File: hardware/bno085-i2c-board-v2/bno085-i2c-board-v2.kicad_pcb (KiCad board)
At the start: 2 copper layers, 13 parts, among them J1 Conn_01x01_Pin, J2 Conn_01x01_Pin, J3 Conn_01x01_Pin, J4 Conn_01x01_Pin, J5 Conn_01x01_Pin, J6 Conn_01x01_Pin

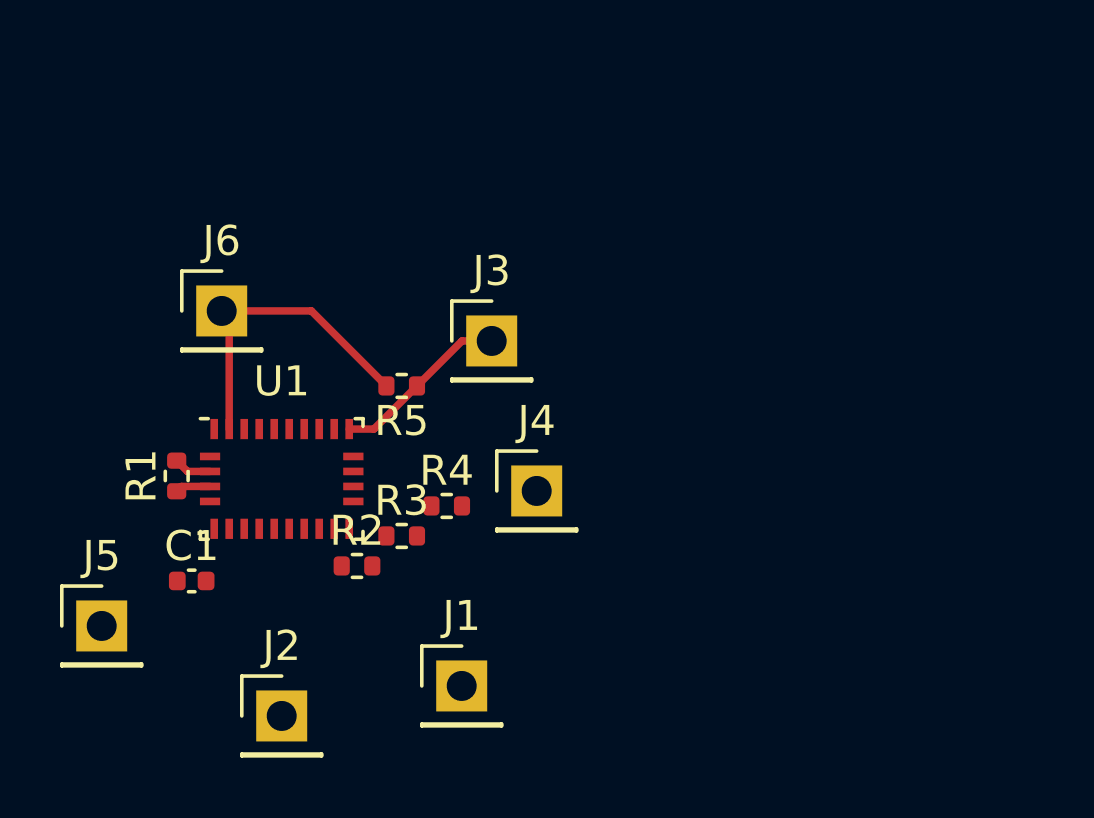
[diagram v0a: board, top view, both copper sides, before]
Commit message: pcb
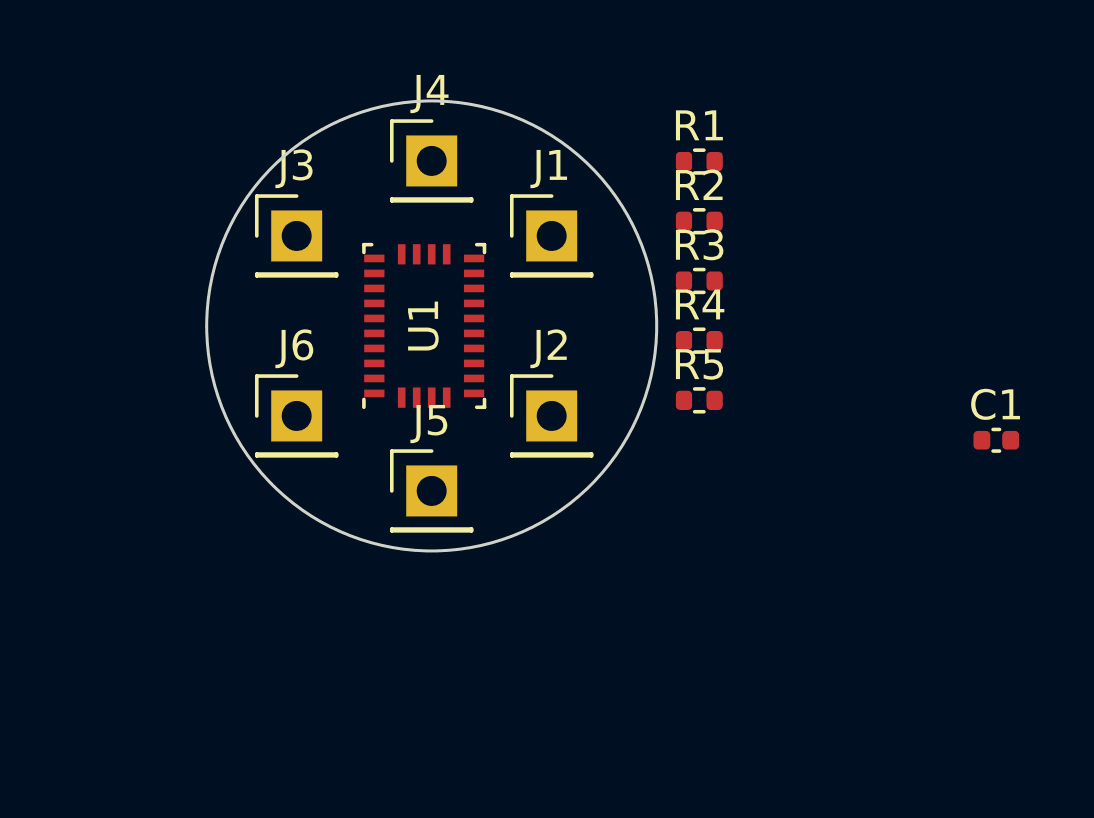
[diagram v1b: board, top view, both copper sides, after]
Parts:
- moved C1 27.2 mm to (188.8, 103.8)
- moved R1 20.3 mm to (178.9, 94.5), turned to 0 degrees
- moved R2 16.2 mm to (178.9, 96.5)
- moved J1 15.3 mm to (174.0, 97.0)
- moved J2 13.5 mm to (174.0, 103.0)
- moved R3 13.1 mm to (178.9, 98.5)
- moved J5 11.9 mm to (170.0, 105.5)
- moved J4 11.5 mm to (170.0, 94.5)
- moved R4 10.1 mm to (178.9, 100.5)
- moved R5 9.93 mm to (178.9, 102.5), turned to 0 degrees
- moved J3 7.38 mm to (165.5, 97.0)
- moved U1 6.97 mm to (169.8, 100.0), turned to 90 degrees
- moved J6 4.30 mm to (165.5, 103.0)
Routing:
- net +3.3V: track 11.8 -> 0.00 mm
- net Net-(J3-Pin_1): track 5.97 -> 0.00 mm
- net Net-(U1-BOOTN): track 1.18 -> 0.00 mm
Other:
- board outline added: 15 x 15 mm
